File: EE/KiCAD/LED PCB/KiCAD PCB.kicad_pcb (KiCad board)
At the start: 2 copper layers, 55.9 x 55.9 mm, 33 parts

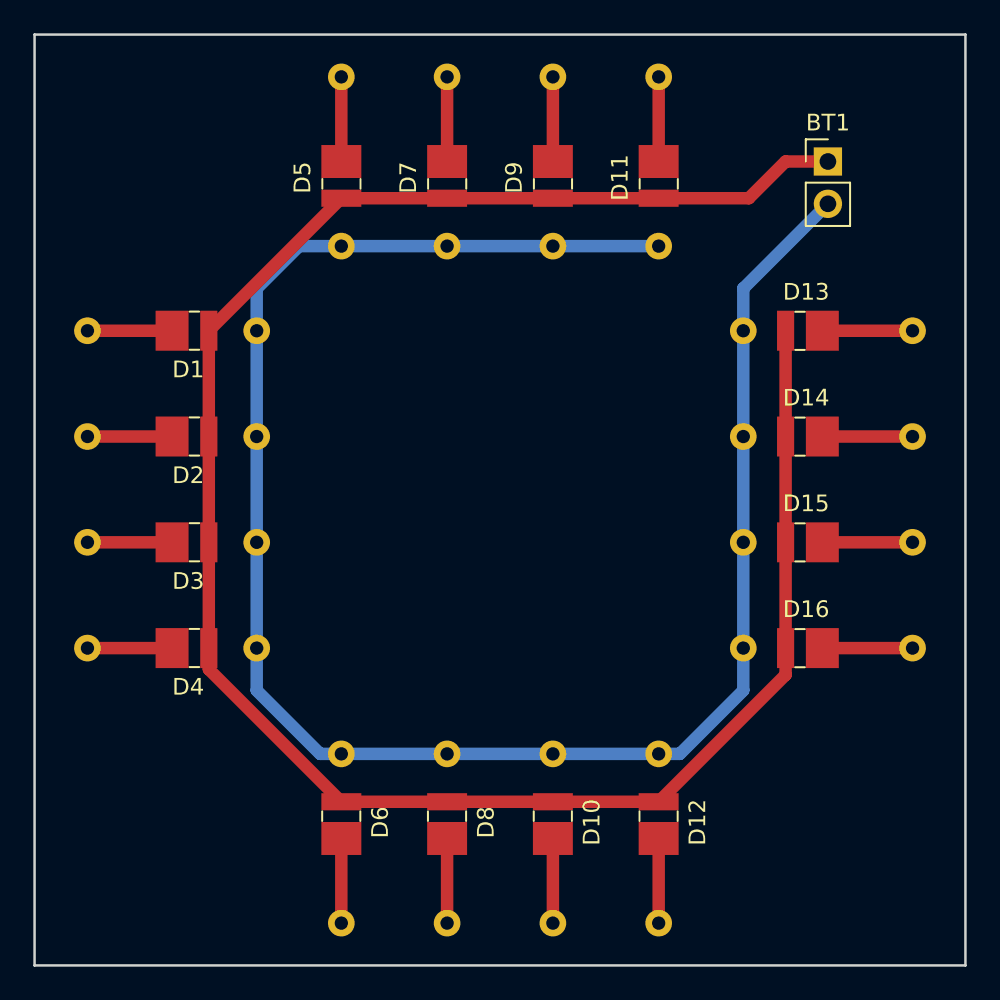
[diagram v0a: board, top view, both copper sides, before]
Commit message: Camera Housing Changes
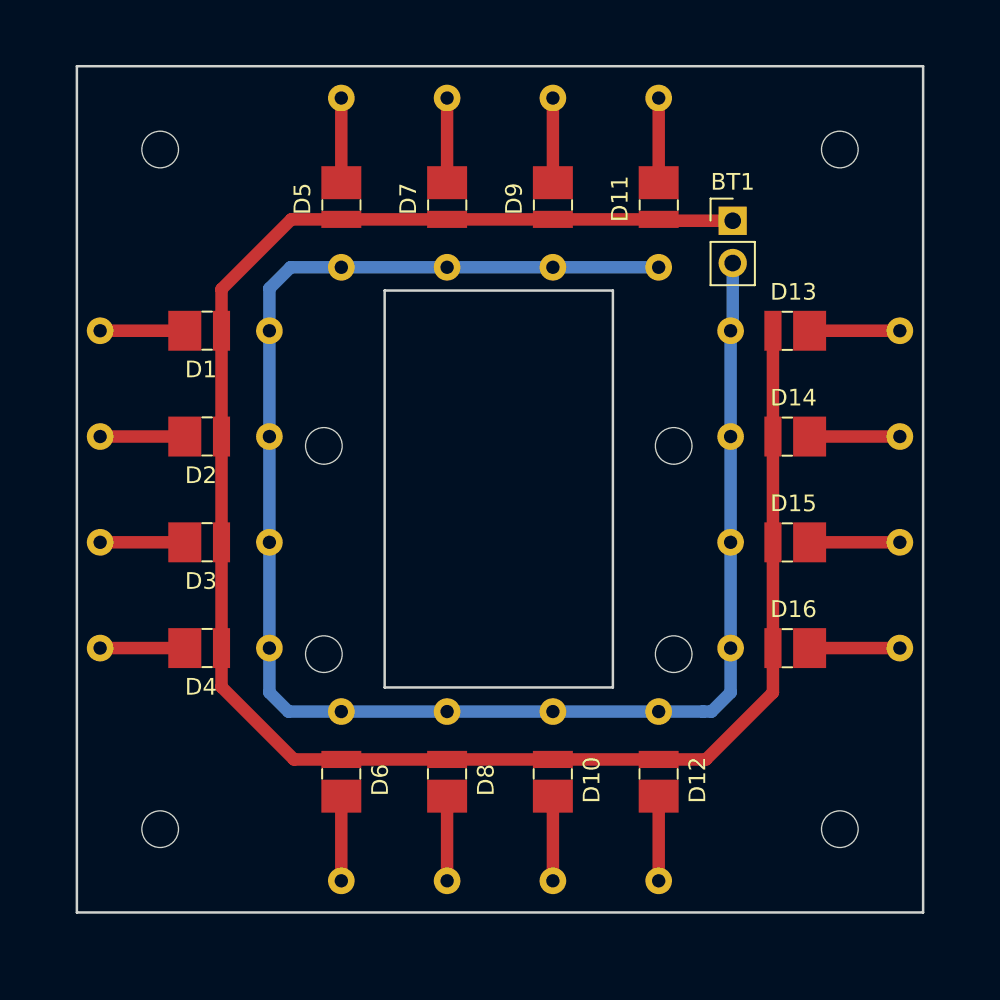
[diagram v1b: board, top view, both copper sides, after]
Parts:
- moved BT1 6.73 mm to (132.1, 70.9)
- moved D10 2.54 mm to (121.3, 104.5)
- moved D12 2.54 mm to (127.6, 104.5)
- moved D6 2.54 mm to (108.6, 104.5)
- moved D8 2.54 mm to (114.9, 104.5)
- moved R10 2.54 mm to (121.3, 100.3)
- moved R12 2.54 mm to (127.6, 100.3)
- moved R6 2.54 mm to (108.6, 100.3)
- moved R8 2.54 mm to (114.9, 100.3)
- moved D11 1.27 mm to (127.6, 69.4)
- moved D5 1.27 mm to (108.6, 69.4)
- moved D7 1.27 mm to (114.9, 69.4)
- moved D9 1.27 mm to (121.3, 69.4)
- moved R11 1.27 mm to (127.6, 73.7)
- moved R5 1.27 mm to (108.6, 73.7)
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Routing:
- net Net-(BT1-Pad2): track 113.0 -> 102.6 mm
- net Net-(BT1-Pad1): track 124.3 -> 115.5 mm
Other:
- board size 55.9 x 55.9 mm -> 50.8 x 50.8 mm
